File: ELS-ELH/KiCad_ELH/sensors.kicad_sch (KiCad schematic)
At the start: 23 parts, among them J10 COM CTR-MAIN, J2 MOSFETS MAIN, J4 Pressure Transducer, J7 Sensors

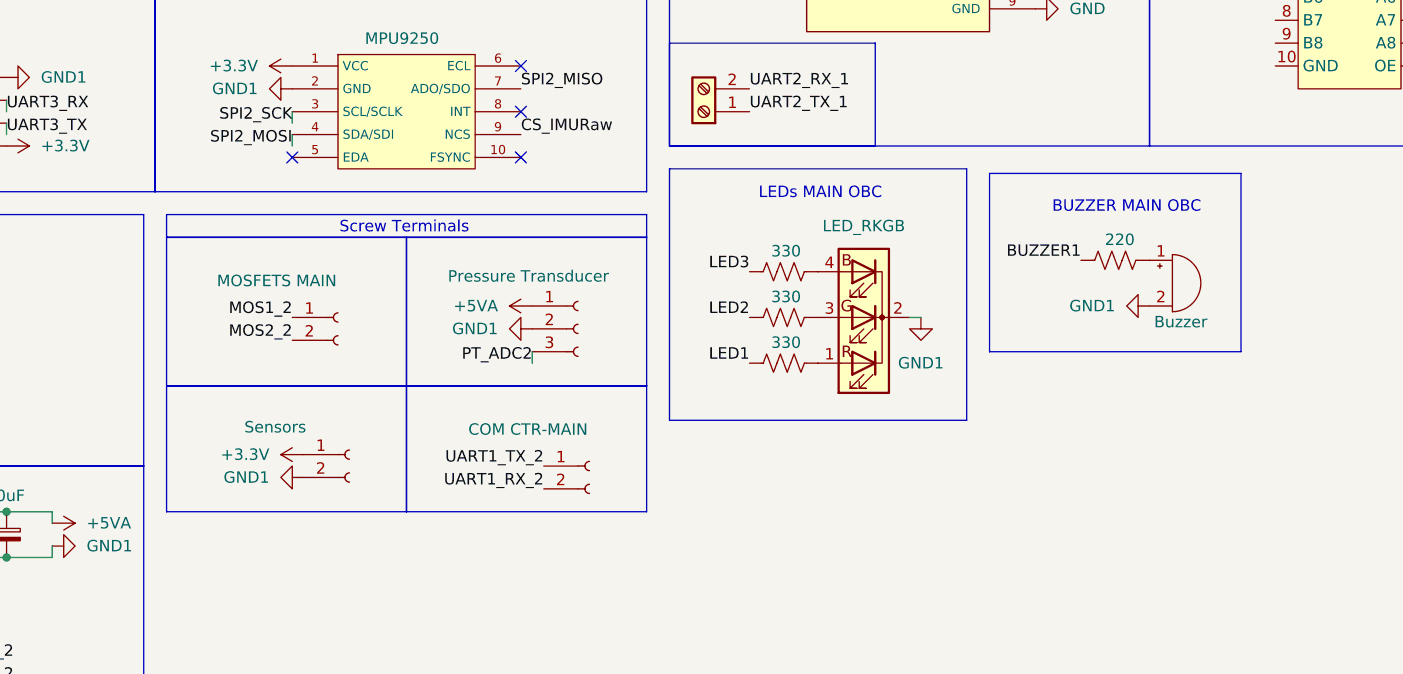
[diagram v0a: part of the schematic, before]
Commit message: Components preliminar distribution
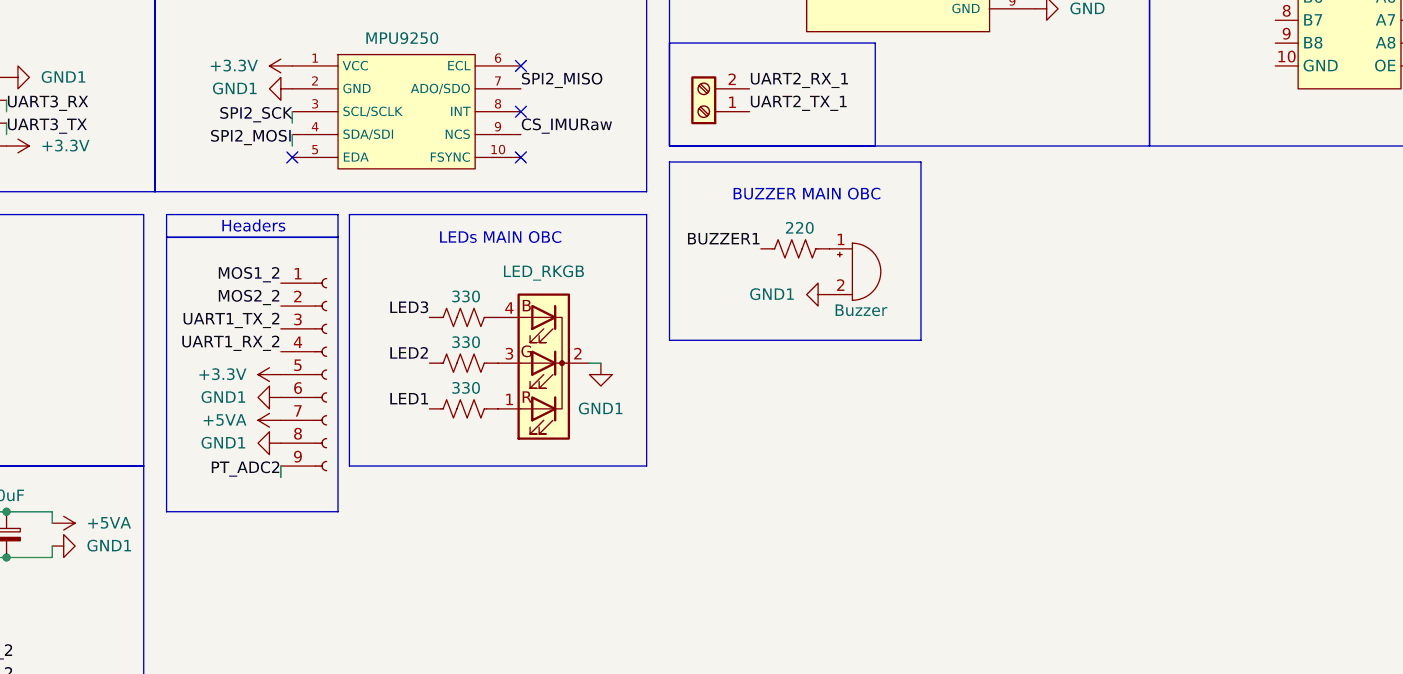
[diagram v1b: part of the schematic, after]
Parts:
- removed J10: COM CTR-MAIN, ELH_Library:2Pin Header, symbol Connector:Conn_01x02_Socket
- removed J2: MOSFETS MAIN, ELH_Library:2Pin Header, symbol Connector:Conn_01x02_Socket
- removed J4: Pressure Transducer, ELH_Library:3Pin Header, symbol Connector:Conn_01x03_Socket
- removed J7: Sensors, ELH_Library:2Pin Header, symbol Connector:Conn_01x02_Socket
- added J11: Conn_01x09_Socket, Connector_Hirose:Hirose_DF13-09P-1.25DSA_1x09_P1.25mm_Vertical, symbol Connector:Conn_01x09_Socket
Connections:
- net +3.3V: now also J11.5 (Pin_5)
- net +5VA: now also J11.7 (Pin_7)
- net GND1: now also J11.6 (Pin_6), J11.8 (Pin_8)
- net MOS1_2: now also J11.1 (Pin_1)
- net MOS2_2: now also J11.2 (Pin_2)
- net PT_ADC2: now also J11.9 (Pin_9)
- net UART1_RX_2: now also J11.4 (Pin_4)
- net UART1_TX_2: now also J11.3 (Pin_3)
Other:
- note added: "Headers"
- note removed: "Screw Terminals"
